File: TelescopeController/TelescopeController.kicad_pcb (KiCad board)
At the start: 2 copper layers, 122.4 x 74 mm, 87 parts, among them J1 PJ-102BH, J10 Screw_Terminal_01x02, J2 RCJ-041, J3 RCJ-041, J4 RCJ-041, J5 Conn_01x03_Pin, J6 Screw_Terminal_01x02, J7 Screw_Terminal_01x02, J8 Screw_Terminal_01x02, J9 Screw_Terminal_01x02, Q1 DMN63D8LW-13, Q2 AO3423, Q3 DMN63D8LW-13, Q4 AO3423, Q5 DMN63D8LW-13, Q6 AO3423, Q7 DMN63D8LW-13, Q8 AO3423

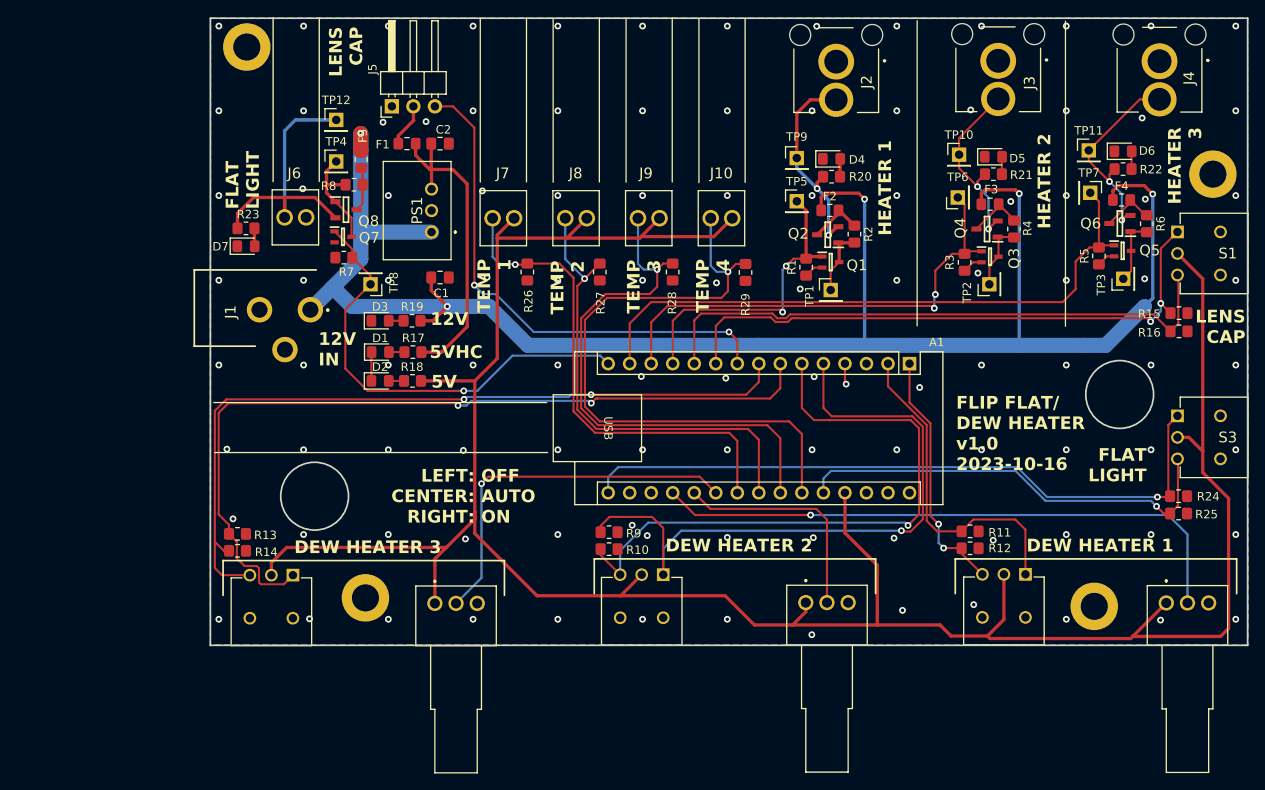
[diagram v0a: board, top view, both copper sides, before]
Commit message: add telescope controller v2
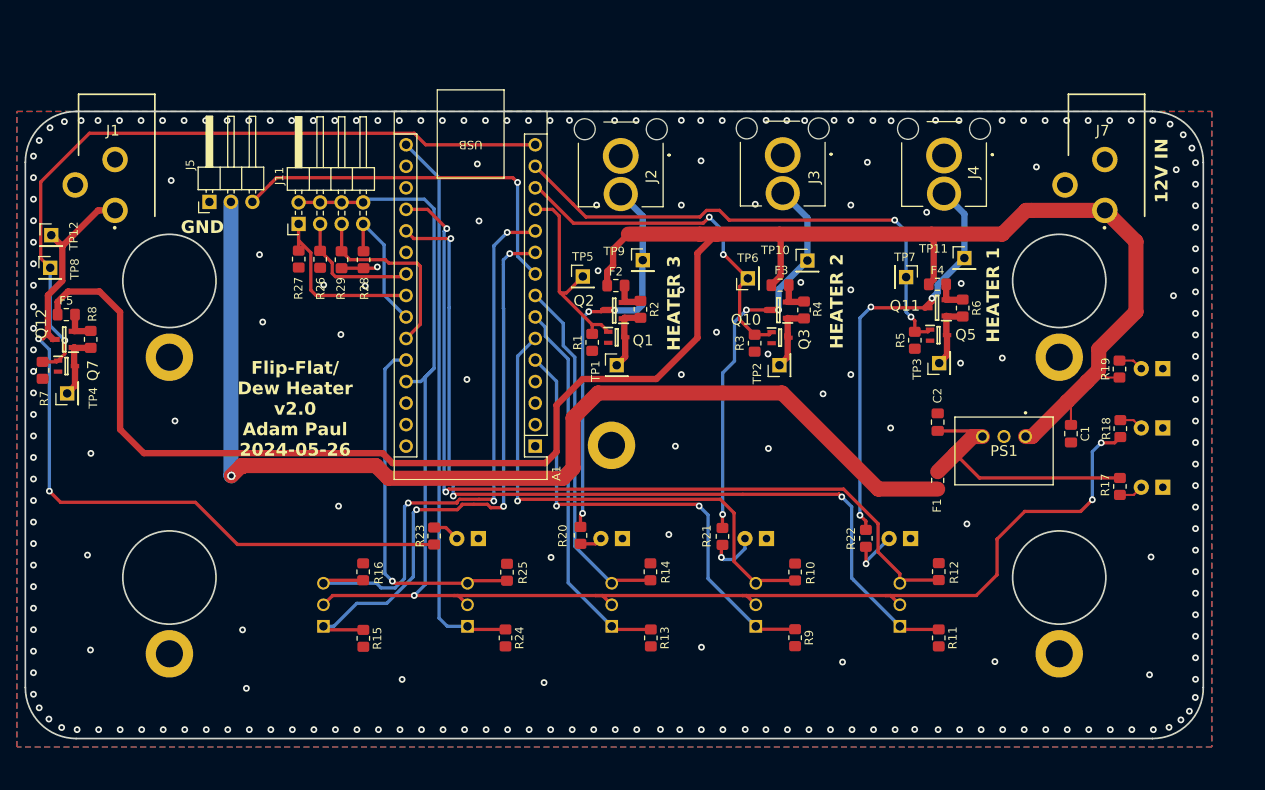
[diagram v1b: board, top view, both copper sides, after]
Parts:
- removed D1, D2, D3, D4, D5, D6, D7: SML-LX0805GC-TR, LED_SMD:LED_0805_2012Metric_Pad1.15x1.40mm_HandSolder
- removed J10, J6, J8, J9: Screw_Terminal_01x02, OSTVN02A150:OSTVN02A150
- removed Q4, Q6, Q8: AO3423, AO3423:SOT95P280X125-3N
- removed the REF** at (84.0, 148.0)
- removed the REF** at (170.0, 149.0)
- removed the REF** at (184.0, 98.0)
- removed the REF** at (70.0, 83.0)
- removed S1, S2, S3, S5, S6: AS1E-5M-10-Z, AS1E-5M-10-Z:AS1E5M10Z
- removed VR1, VR4, VR5: PTD901-1015K-B103, PTD901-1015K-B103:PTD9011015KB103
- added D10: LED, LED_THT:LED_D3.0mm, B.Cu at (178.1, 134.9)
- added D11: LED, LED_THT:LED_D3.0mm, B.Cu at (178.1, 121.0)
- added D12: LED, LED_THT:LED_D3.0mm, B.Cu at (114.3, 141.0)
- added D13: LED, LED_THT:LED_D3.0mm, B.Cu at (97.3, 141.0)
- added D14: LED, LED_THT:LED_D3.0mm, B.Cu at (178.1, 128.0)
- added D8: LED, LED_THT:LED_D3.0mm, B.Cu at (148.3, 141.0)
- added D9: LED, LED_THT:LED_D3.0mm, B.Cu at (131.3, 141.0)
- added J11: Conn_02x04_Counter_Clockwise, Connector_PinHeader_2.54mm:PinHeader_2x04_P2.54mm_Horizontal, F.Cu at (76.1, 103.9)
- added Q10: DMP3099L-7, DMP3099L-7:SOT96P240X115-3N, F.Cu at (132.7, 114.0)
- added Q11: DMP3099L-7, DMP3099L-7:SOT96P240X115-3N, F.Cu at (151.4, 113.8)
- added Q12: DMP3099L-7, DMP3099L-7:SOT96P240X115-3N, F.Cu at (48.5, 117.5)
- added REF**: MountingHole_3.2mm_M3_DIN965_Pad, MountingHole:MountingHole_3.2mm_M3_DIN965_Pad, F.Cu at (165.9, 154.6)
- added REF**: MountingHole_3.2mm_M3_DIN965_Pad, MountingHole:MountingHole_3.2mm_M3_DIN965_Pad, F.Cu at (60.9, 154.6)
- added REF**: MountingHole_3.2mm_M3_DIN965_Pad, MountingHole:MountingHole_3.2mm_M3_DIN965_Pad, F.Cu at (165.9, 119.6)
- added REF**: MountingHole_3.2mm_M3_DIN965_Pad, MountingHole:MountingHole_3.2mm_M3_DIN965_Pad, F.Cu at (113.0, 130.0)
- added REF**: MountingHole_3.2mm_M3_DIN965_Pad, MountingHole:MountingHole_3.2mm_M3_DIN965_Pad, F.Cu at (60.9, 119.6)
- added S10: AS1E-2M-10-Z, AS1E-2M-10-Z:AS1E2M10Z, B.Cu at (79.0, 151.4)
- added S4: AS1E-2M-10-Z, AS1E-2M-10-Z:AS1E2M10Z, B.Cu at (130.1, 151.4)
- added S7: AS1E-2M-10-Z, AS1E-2M-10-Z:AS1E2M10Z, B.Cu at (113.1, 151.4)
- added S8: AS1E-2M-10-Z, AS1E-2M-10-Z:AS1E2M10Z, B.Cu at (147.1, 151.4)
- added S9: AS1E-2M-10-Z, AS1E-2M-10-Z:AS1E2M10Z, B.Cu at (96.0, 151.4)
- F2, F3, F4, F5: value 1A -> 1.5A
- J7: value Screw_Terminal_01x02 -> PJ-102BH; footprint OSTVN02A150:OSTVN02A150 -> PJ-102BH:PJ-102AH
- Q2: value AO3423 -> DMP3099L-7; footprint AO3423:SOT95P280X125-3N -> DMP3099L-7:SOT96P240X115-3N
- R17, R18: value 140R -> 300R
- R19, R20, R21, R22, R23: value 490R -> 1k
- R2, R4, R6, R8: value 100R -> 1k
- moved R15 103.6 mm to (83.8, 152.8), turned to -90 degrees
- moved R16 100.4 mm to (83.7, 144.9), turned to 90 degrees
- moved R17 84.9 mm to (173.0, 134.8), turned to -90 degrees
- moved R18 83.7 mm to (173.1, 128.0), turned to 90 degrees
- moved R19 83.7 mm to (173.0, 121.0), turned to 90 degrees
- moved R24 81.2 mm to (100.5, 152.7), turned to -90 degrees
- moved R25 79.6 mm to (100.7, 145.0), turned to 90 degrees
- moved C1 76.7 mm to (167.2, 128.6), turned to -90 degrees
- moved F1 74.2 mm to (151.5, 134.1), turned to -90 degrees
- moved PS1 74.1 mm to (161.9, 129.0), turned to 180 degrees
- moved J7 68.1 mm to (166.9, 99.3)
- moved C2 67.3 mm to (151.5, 127.3), turned to 90 degrees
- moved R21 53.4 mm to (126.1, 140.8), turned to -90 degrees
- moved R22 53.1 mm to (143.1, 141.0), turned to -90 degrees
- moved R20 51.7 mm to (109.4, 140.6), turned to -90 degrees
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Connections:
- A1 pad 1: /HEATER1_OFF -> unconnected-(A1-D1/TX-Pad1)
- A1 pad 19: Net-(A1-A0) -> /HEATER1_OFF
- A1 pad 2: /HEATER1_ON -> unconnected-(A1-D0/RX-Pad2)
- A1 pad 20: Net-(A1-A1) -> /HEATER1_ON
- A1 pad 21: Net-(A1-A2) -> unconnected-(A1-A2-Pad21)
- F2 pad 2: Net-(Q2-D) -> Net-(Q2-S)
- J1 pad 1: +12V -> /12V_SWITCHING3/OUT
- J7 pad 1: /Thermistor/AOUT -> +12V
- J7 pad 2: +5V -> GND
- Q2 pad 2: /12V_SWITCHING/OUT -> Net-(Q2-S)
- Q2 pad 3: Net-(Q2-D) -> /12V_SWITCHING/OUT
- R2 pad 1: Net-(Q2-D) -> Net-(Q2-S)
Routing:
- net Net-(J5-Pin_2): track 5.17 -> 129.3 mm, vias 0 -> 1
- net +5V: track 298.8 -> 183.8 mm, vias 0 -> 3
- net /HEATER1_OFF: track 29.7 -> 102.7 mm
- net Net-(A1-A0): track 70.9 -> 0.00 mm, vias 1 -> 0
- net /HEATER1_ON: track 39.0 -> 105.3 mm, vias 0 -> 3
- net /12V_SWITCHING3/OUT: track 34.3 -> 89.6 mm, vias 0 -> 2
- net /HEATER3_ON: track 98.2 -> 45.0 mm, vias 2 -> 0
- net /Thermistor3/AOUT: track 75.1 -> 22.5 mm, vias 1 -> 0
- net /HEATER3_OFF: track 93.0 -> 42.4 mm, vias 2 -> 0
- net /Thermistor2/AOUT: track 64.6 -> 16.3 mm, vias 1 -> 0
- net Net-(A1-A2): track 44.1 -> 0.00 mm, vias 1 -> 0
- net /Thermistor/AOUT: track 57.9 -> 15.4 mm, vias 1 -> 0
- net /Thermistor1/AOUT: track 55.6 -> 21.1 mm, vias 1 -> 0
- net /12V_SWITCHING3/IN: track 53.8 -> 85.8 mm
- net Net-(A1-A1): track 26.8 -> 0.00 mm
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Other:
- board size 122.4 x 74 mm -> 139 x 74 mm
- board text added: "1"
- board text added: "2"
- board text added: "3"
- board text added: "Flip-Flat/ Dew Heater v2.0 Adam Paul 2024-05-26"
- board text added: "GND"
- board text added: "HEATER"
- board text added: "LIGHT"
- board text added: "USB"
- board text removed: "5VHC"
- board text removed: "DEW HEATER 1"
- board text removed: "DEW HEATER 2"
- board text removed: "DEW HEATER 3"
- board text removed: "FLAT LIGHT"
- board text removed: "FLIP FLAT/ DEW HEATER v1.0 2023-10-16"
- board text removed: "LEFT: CENTER: RIGHT:"
- board text removed: "OFF AUTO ON"
- board text removed: "TEMP 1"
- board text removed: "TEMP 2"
- board text removed: "TEMP 3"
- board text removed: "TEMP 4"
